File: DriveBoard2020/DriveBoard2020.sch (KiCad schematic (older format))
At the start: 66 parts, among them SW0 SW_SPST, SW1 SW_Push, SW3 SW_Push, SW5 SW_Push, SW7 SW_Push, SW8 SW_Push, SW9 SW_Push, U1 MAX_3232, U2 MAX_3232, U3 OKI, U4 TM4C129E_Launchpad, U5 MAX_3232, U6 OKI, U8 LDD-1500L

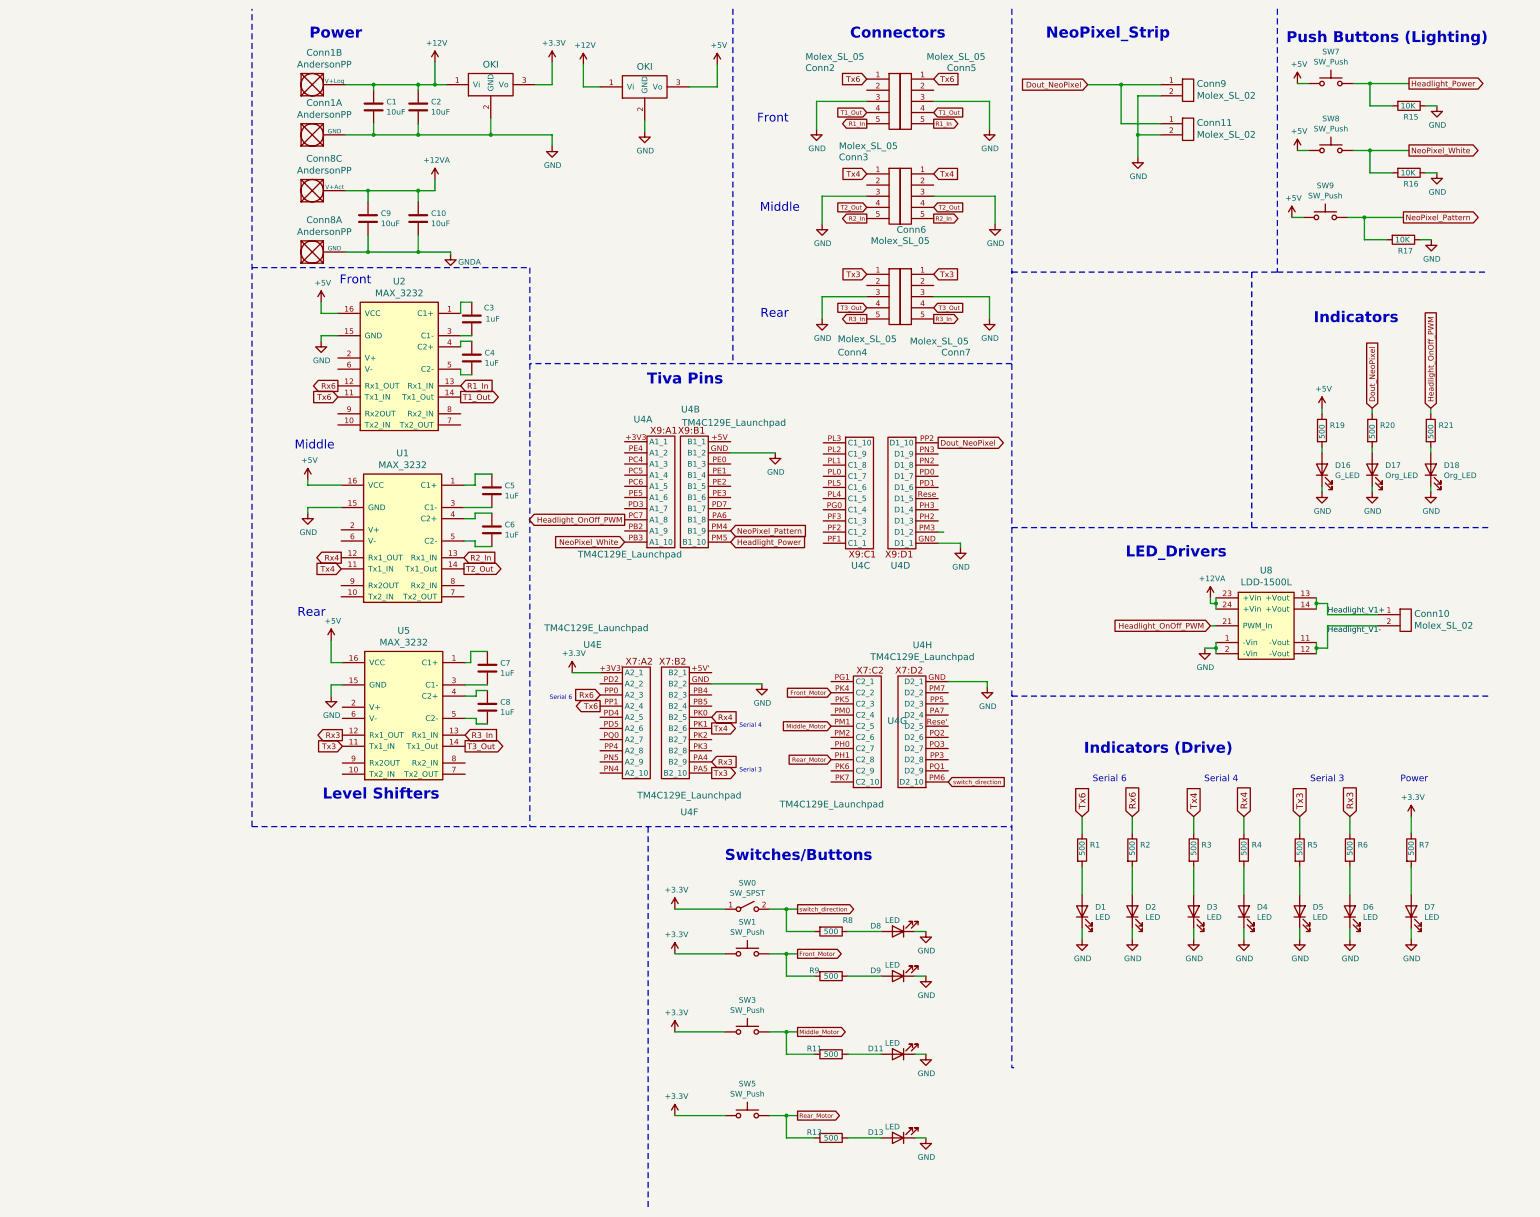
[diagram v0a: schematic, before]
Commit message: Worked on grids
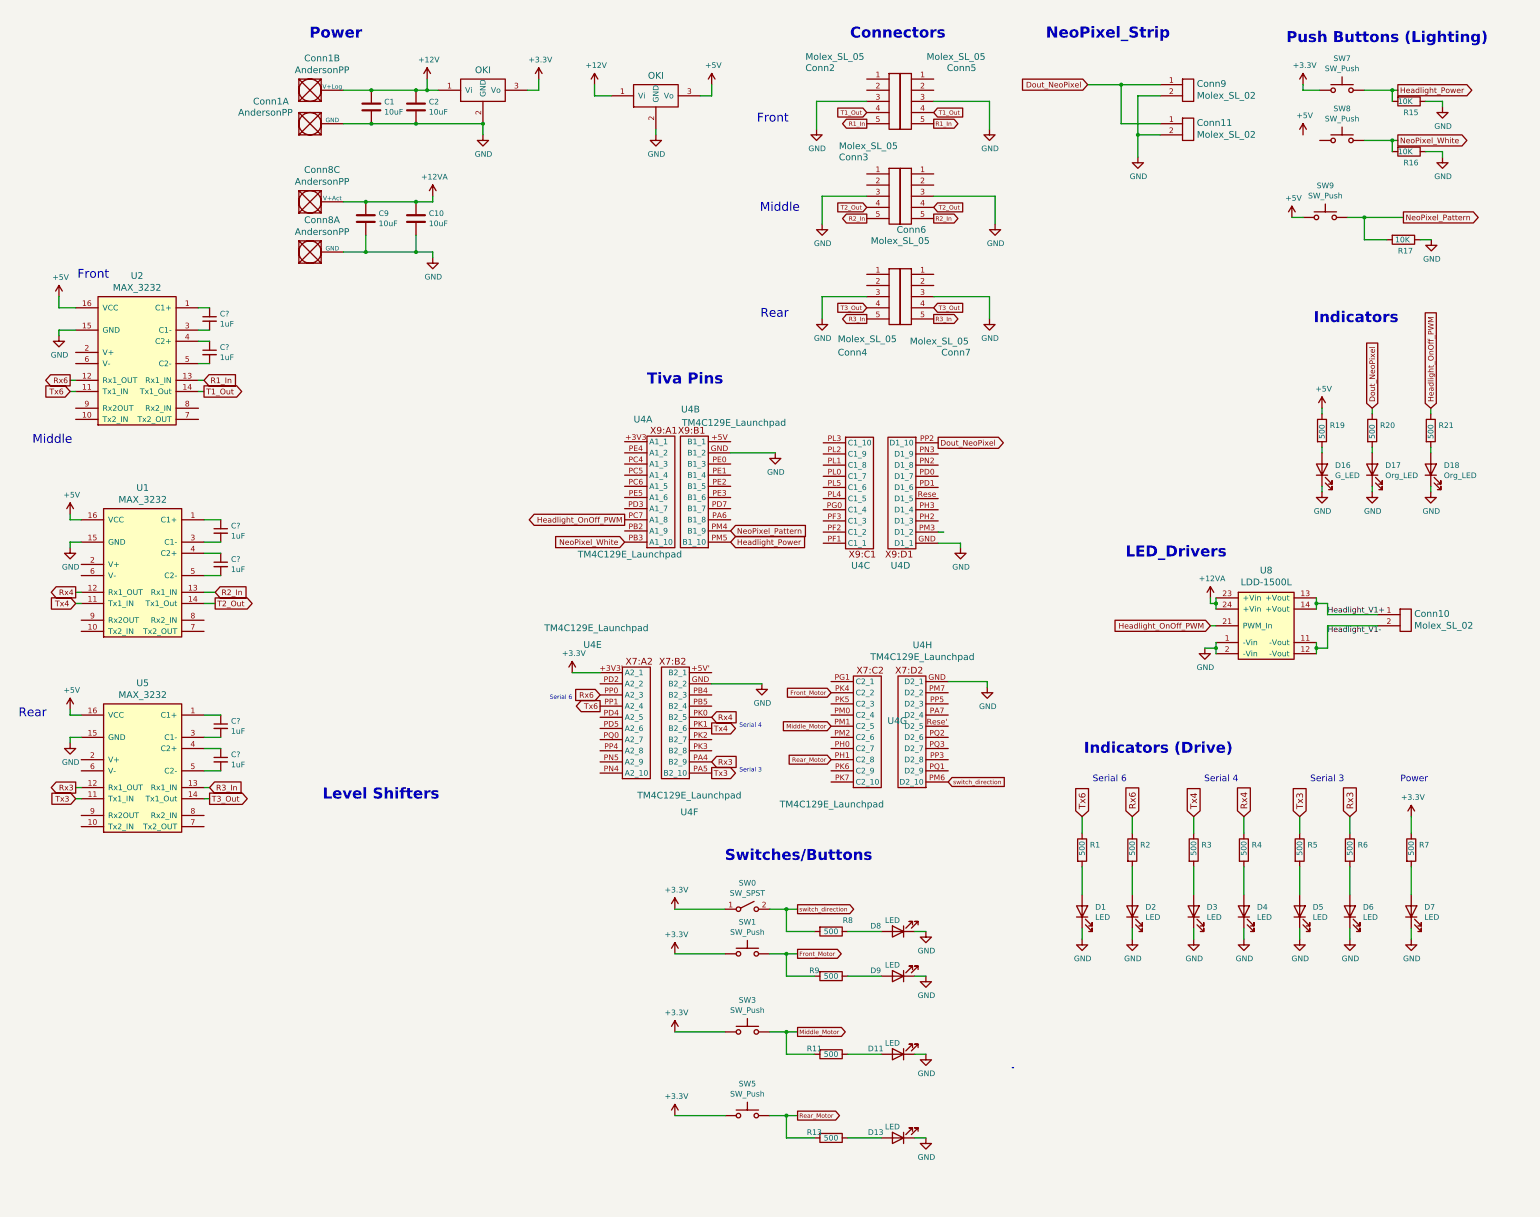
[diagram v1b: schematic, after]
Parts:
- removed C3, C4, C5, C6, C7, C8: 1uF, Capacitor_SMD:C_0603_1608Metric_Pad1.05x0.95mm_HandSolder, symbol Device:C
- added C? (x6): 1uF, symbol Device:C_Small
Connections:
- net GNDA is gone; now on net GND: C10.2, C9.2, Conn8.1 (GND)
- net +3V3: now also SW7.1
- net +5V: no longer SW7.1, SW8.1
- net Tx3: no longer Conn4.1, Conn7.1
- net Tx4: no longer Conn3.1, Conn6.1
- net Tx6: no longer Conn2.1, Conn5.1
- net at U1.1 (C1+): now also C?.1
- net at U1.3 (C1-): now also C?.2
- net at U1.4 (C2+): now also C?.1
- net at U1.5 (C2-): now also C?.2
- net at U2.3 (C1-): now also C?.2
- net at U2.1 (C1+): now also C?.1
- net at U2.4 (C2+): now also C?.1
- net at U2.5 (C2-): now also C?.2
- net at U5.1 (C1+): now also C?.1
- net at U5.3 (C1-): now also C?.2
- net at U5.4 (C2+): now also C?.1
- net at U5.5 (C2-): now also C?.2
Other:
- moved on the sheet: C1, C10, C2, C9, Conn1A, Conn1B, Conn8A, Conn8C, R15, R16, SW7, SW8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
